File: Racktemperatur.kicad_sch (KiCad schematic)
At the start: 24 parts, among them J1 Conn_01x03, J2 Conn_01x03, J3 Barrel_Jack_MountingPin, J4 Screw_Terminal_01x02, Q1 IRLZ44N, U1 74HC595, U2 74HC595, U3 DS18B20, U4 L7805

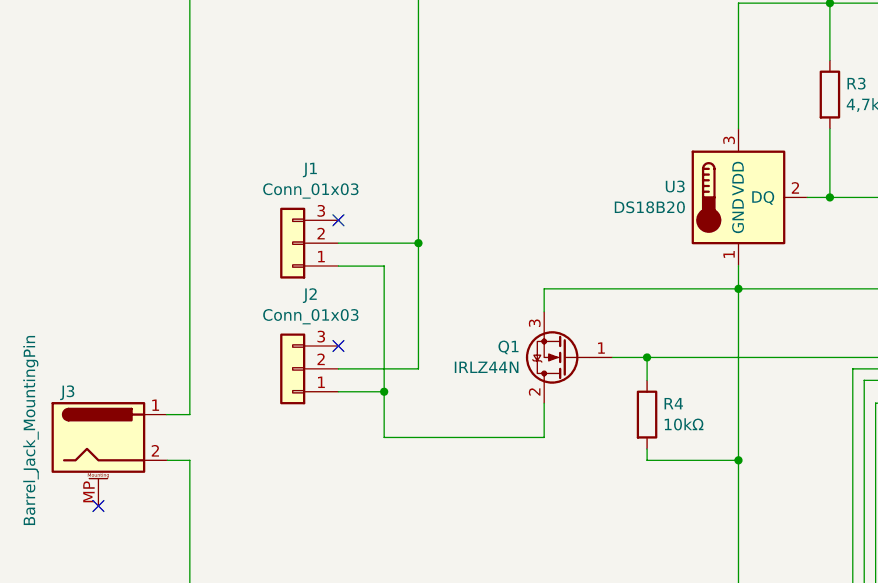
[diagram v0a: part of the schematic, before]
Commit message: v1.6
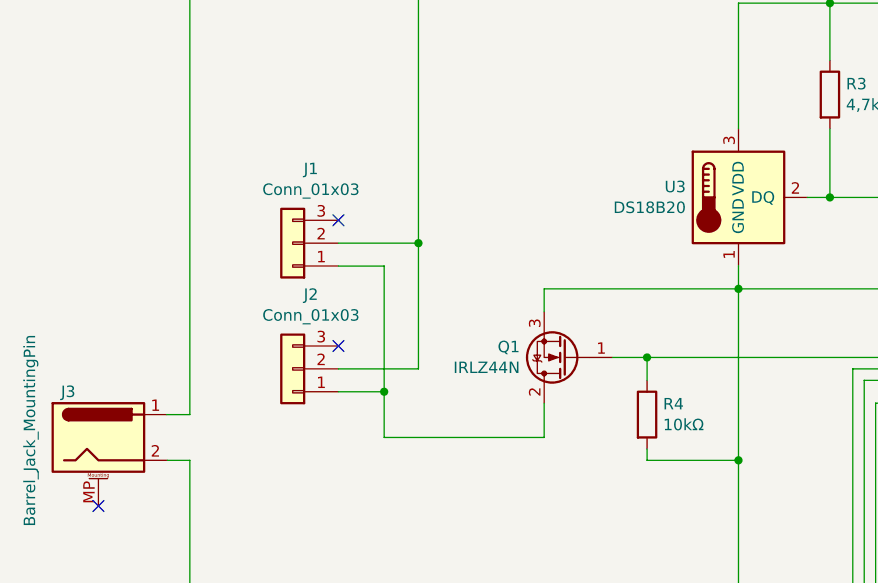
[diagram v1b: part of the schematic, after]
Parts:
- C1, C2: footprint Capacitor_SMD:C_0805_2012Metric_Pad1.15x1.40mm_HandSolder -> Capacitor_SMD:C_0805_2012Metric_Pad1.18x1.45mm_HandSolder
- R1, R2, R3, R4, R5, R6, R7: footprint Resistor_SMD:R_0805_2012Metric_Pad1.15x1.40mm_HandSolder -> Resistor_SMD:R_0805_2012Metric_Pad1.20x1.40mm_HandSolder
